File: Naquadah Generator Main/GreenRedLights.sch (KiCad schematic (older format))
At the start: 4 parts, among them J2 Conn_01x02, J5 Conn_01x02, Q1 BC337

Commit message: Before changing BOM
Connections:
- net labels added: +5V, GND
- net labels removed: 5V, VGND
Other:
- moved on the sheet: R33
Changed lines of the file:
@@
 $Descr A4 11693 8268
 encoding utf-8
-Sheet 11 14
+Sheet 9 10
 Title ""
 Date ""
@@
 $EndDescr
 Wire Wire Line
-	5450 4750 5400 4750
+	5450 4550 5450 4650
 Wire Wire Line
-	5450 4550 5450 4750
-Wire Wire Line
-	4650 4350 4850 4350
+	4650 4350 4750 4350
 Text HLabel 4650 4350 0    50   Input ~ 0
 SIGNAL
@@
 L Device:R R?
 U 1 1 5E9E70EB
-P 5000 4350
+P 4900 4350
 AR Path="/5E9E5DDE/5E9E70EB" Ref="R?"  Part="1"
 AR Path="/5E9E304D/5E9E70EB" Ref="R?"  Part="1"
@@
 AR Path="/5EA4676F/5E9E70EB" Ref="R33"  Part="1"
 AR Path="/5EA46A2B/5E9E70EB" Ref="R34"  Part="1"
-F 0 "R33" V 4793 4350 50  0000 C CNN
-F 1 "2.7k" V 4884 4350 50  0000 C CNN
-F 2 "Resistor_THT:R_Axial_DIN0207_L6.3mm_D2.5mm_P10.16mm_Horizontal" V 4930 4350 50  0001 C CNN
-F 3 "~" H 5000 4350 50  0001 C CNN
-	1    5000 4350
+F 0 "R33" V 4800 4350 50  0000 C CNN
+F 1 "2.7k" V 5000 4350 50  0000 C CNN
+F 2 "Resistor_THT:R_Axial_DIN0207_L6.3mm_D2.5mm_P10.16mm_Horizontal" V 4830 4350 50  0001 C CNN
+F 3 "~" H 4900 4350 50  0001 C CNN
+	1    4900 4350
 	0    1    1    0
 $EndComp
-Text GLabel 5400 4750 0    50   Input ~ 0
-VGND
 $Comp
 L Transistor_BJT:BC337 Q?
@@
 	1    0    0    -1
 $EndComp
-Text GLabel 5250 3650 0    50   Input ~ 0
-5V
 $Comp
 L Connector_Generic:Conn_01x02 J5
@@
 AR Path="/5EA4676F/5EAB251D" Ref="J6"  Part="1"
 AR Path="/5EA46A2B/5EAB251D" Ref="J?"  Part="1"
-F 0 "J6" H 6000 3700 50  0000 C CNN
-F 1 "Conn_01x02" H 6150 3800 50  0000 C CNN
+F 0 "J6" H 5900 3800 50  0000 L CNN
+F 1 "Conn_01x02" H 5900 3700 50  0000 L CNN
 F 2 "Connector_Wire:SolderWirePad_1x02_P3.81mm_Drill1.2mm" H 5800 3800 50  0001 C CNN
 F 3 "~" H 5800 3800 50  0001 C CNN
@@
 AR Path="/5EA4676F/5EA51394" Ref="J3"  Part="1"
 AR Path="/5EA46A2B/5EA51394" Ref="J4"  Part="1"
-F 0 "J3" H 5600 3800 50  0000 C CNN
-F 1 "Conn_01x02" H 5450 3900 50  0000 C CNN
+F 0 "J3" H 5650 3800 50  0000 R CNN
+F 1 "Conn_01x02" H 5650 3900 50  0000 R CNN
 F 2 "Connector_Wire:SolderWirePad_1x02_P3.81mm_Drill1.2mm" H 5100 3900 50  0001 C CNN
 F 3 "~" H 5100 3900 50  0001 C CNN
@@
 Wire Wire Line
 	5450 3900 5450 4150
-Text GLabel 5650 4050 2    50   Input ~ 0
-5V
 Wire Wire Line
-	5600 3900 5600 4050
+	5350 3750 5350 3800
 Wire Wire Line
-	5600 4050 5650 4050
+	5600 3900 5550 3900
 Wire Wire Line
-	5250 3650 5300 3650
+	5550 3900 5550 3750
+$Comp
+L power:+5V #PWR?
+U 1 1 5EC1DBF9
+P 5350 3750
+AR Path="/5EA45E37/5EC1DBF9" Ref="#PWR?"  Part="1"
+AR Path="/5EA4676F/5EC1DBF9" Ref="#PWR?"  Part="1"
+F 0 "#PWR?" H 5350 3600 50  0001 C CNN
+F 1 "+5V" H 5365 3923 50  0000 C CNN
+F 2 "" H 5350 3750 50  0001 C CNN
+F 3 "" H 5350 3750 50  0001 C CNN
+	1    5350 3750
+	1    0    0    -1
+$EndComp
+$Comp
+L power:+5V #PWR?
+U 1 1 5EC1E71E
+P 5550 3750
+AR Path="/5EA45E37/5EC1E71E" Ref="#PWR?"  Part="1"
+AR Path="/5EA4676F/5EC1E71E" Ref="#PWR?"  Part="1"
+F 0 "#PWR?" H 5550 3600 50  0001 C CNN
+F 1 "+5V" H 5565 3923 50  0000 C CNN
+F 2 "" H 5550 3750 50  0001 C CNN
+F 3 "" H 5550 3750 50  0001 C CNN
+	1    5550 3750
+	1    0    0    -1
+$EndComp
 Wire Wire Line
-	5300 3650 5300 3800
+	5350 3800 5300 3800
+$Comp
+L power:GND #PWR?
+U 1 1 5EC21498
+P 5450 4650
+AR Path="/5EA45E37/5EC21498" Ref="#PWR?"  Part="1"
+AR Path="/5EA4676F/5EC21498" Ref="#PWR?"  Part="1"
+F 0 "#PWR?" H 5450 4400 50  0001 C CNN
+F 1 "GND" H 5455 4477 50  0000 C CNN
+F 2 "" H 5450 4650 50  0001 C CNN
+F 3 "" H 5450 4650 50  0001 C CNN
+	1    5450 4650
+	1    0    0    -1
+$EndComp
+Wire Wire Line
+	5050 4350 5150 4350
 $EndSCHEMATC

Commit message: Changed name of libraries to remove underscore
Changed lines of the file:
@@
 $Descr A4 11693 8268
 encoding utf-8
-Sheet 9 10
+Sheet 9 11
 Title ""
 Date ""
@@
 AR Path="/5EA4676F/5E9E70EB" Ref="R33"  Part="1"
 AR Path="/5EA46A2B/5E9E70EB" Ref="R34"  Part="1"
-F 0 "R33" V 4800 4350 50  0000 C CNN
+AR Path="/5ED17BA0/5ED2A32F/5E9E70EB" Ref="R?"  Part="1"
+AR Path="/5ED17BA0/5ED2A36D/5E9E70EB" Ref="R?"  Part="1"
+F 0 "R?" V 4800 4350 50  0000 C CNN
 F 1 "2.7k" V 5000 4350 50  0000 C CNN
 F 2 "Resistor_THT:R_Axial_DIN0207_L6.3mm_D2.5mm_P10.16mm_Horizontal" V 4830 4350 50  0001 C CNN
@@
 AR Path="/5EA4676F/5EAB722E" Ref="Q2"  Part="1"
 AR Path="/5EA46A2B/5EAB722E" Ref="Q3"  Part="1"
-F 0 "Q2" H 5541 4396 50  0000 L CNN
+AR Path="/5ED17BA0/5ED2A32F/5EAB722E" Ref="Q?"  Part="1"
+AR Path="/5ED17BA0/5ED2A36D/5EAB722E" Ref="Q?"  Part="1"
+F 0 "Q?" H 5541 4396 50  0000 L CNN
 F 1 "BC337" H 5541 4305 50  0000 L CNN
 F 2 "Package_TO_SOT_THT:TO-92_Inline" H 5550 4275 50  0001 L CIN
@@
 AR Path="/5EA4676F/5EAB251D" Ref="J6"  Part="1"
 AR Path="/5EA46A2B/5EAB251D" Ref="J?"  Part="1"
-F 0 "J6" H 5900 3800 50  0000 L CNN
+AR Path="/5ED17BA0/5ED2A32F/5EAB251D" Ref="J?"  Part="1"
+AR Path="/5ED17BA0/5ED2A36D/5EAB251D" Ref="J?"  Part="1"
+F 0 "J?" H 5900 3800 50  0000 L CNN
 F 1 "Conn_01x02" H 5900 3700 50  0000 L CNN
 F 2 "Connector_Wire:SolderWirePad_1x02_P3.81mm_Drill1.2mm" H 5800 3800 50  0001 C CNN
@@
 AR Path="/5EA4676F/5EA51394" Ref="J3"  Part="1"
 AR Path="/5EA46A2B/5EA51394" Ref="J4"  Part="1"
-F 0 "J3" H 5650 3800 50  0000 R CNN
+AR Path="/5ED17BA0/5ED2A32F/5EA51394" Ref="J?"  Part="1"
+AR Path="/5ED17BA0/5ED2A36D/5EA51394" Ref="J?"  Part="1"
+F 0 "J?" H 5650 3800 50  0000 R CNN
 F 1 "Conn_01x02" H 5650 3900 50  0000 R CNN
 F 2 "Connector_Wire:SolderWirePad_1x02_P3.81mm_Drill1.2mm" H 5100 3900 50  0001 C CNN
@@
 AR Path="/5EA45E37/5EC1DBF9" Ref="#PWR?"  Part="1"
 AR Path="/5EA4676F/5EC1DBF9" Ref="#PWR?"  Part="1"
+AR Path="/5ED17BA0/5ED2A32F/5EC1DBF9" Ref="#PWR?"  Part="1"
+AR Path="/5ED17BA0/5ED2A36D/5EC1DBF9" Ref="#PWR?"  Part="1"
 F 0 "#PWR?" H 5350 3600 50  0001 C CNN
 F 1 "+5V" H 5365 3923 50  0000 C CNN
@@
 AR Path="/5EA45E37/5EC1E71E" Ref="#PWR?"  Part="1"
 AR Path="/5EA4676F/5EC1E71E" Ref="#PWR?"  Part="1"
+AR Path="/5ED17BA0/5ED2A32F/5EC1E71E" Ref="#PWR?"  Part="1"
+AR Path="/5ED17BA0/5ED2A36D/5EC1E71E" Ref="#PWR?"  Part="1"
 F 0 "#PWR?" H 5550 3600 50  0001 C CNN
 F 1 "+5V" H 5565 3923 50  0000 C CNN
@@
 AR Path="/5EA45E37/5EC21498" Ref="#PWR?"  Part="1"
 AR Path="/5EA4676F/5EC21498" Ref="#PWR?"  Part="1"
+AR Path="/5ED17BA0/5ED2A32F/5EC21498" Ref="#PWR?"  Part="1"
+AR Path="/5ED17BA0/5ED2A36D/5EC21498" Ref="#PWR?"  Part="1"
 F 0 "#PWR?" H 5450 4400 50  0001 C CNN
 F 1 "GND" H 5455 4477 50  0000 C CNN

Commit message: Partial Update
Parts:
- removed Q1: BC337, Package_TO_SOT_THT:TO-92_Inline, symbol Transistor_BJT:BC337
- added Q1: BCW65ALT1G, Package_TO_SOT_SMD:SOT-23, symbol Frequently_Used:BCW65ALT1G
- R30: renamed from R32; footprint Resistor_THT:R_Axial_DIN0207_L6.3mm_D2.5mm_P10.16mm_Horizontal -> Frequently_Used:0805_2012Metric_HandSolder
- renumbered J2 to J4
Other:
- moved on the sheet: J4, J5
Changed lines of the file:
@@
 $Descr A4 11693 8268
 encoding utf-8
-Sheet 9 11
+Sheet 10 11
 Title ""
 Date ""
@@
 AR Path="/5E9E5DE1/5E9E70EB" Ref="R?"  Part="1"
 AR Path="/5E9E4A6B/5E9E70EB" Ref="R?"  Part="1"
-AR Path="/5EA45E37/5E9E70EB" Ref="R32"  Part="1"
-AR Path="/5EA4676F/5E9E70EB" Ref="R33"  Part="1"
-AR Path="/5EA46A2B/5E9E70EB" Ref="R34"  Part="1"
-AR Path="/5ED17BA0/5ED2A32F/5E9E70EB" Ref="R?"  Part="1"
-AR Path="/5ED17BA0/5ED2A36D/5E9E70EB" Ref="R?"  Part="1"
-F 0 "R?" V 4800 4350 50  0000 C CNN
+AR Path="/5EA45E37/5E9E70EB" Ref="R?"  Part="1"
+AR Path="/5EA4676F/5E9E70EB" Ref="R?"  Part="1"
+AR Path="/5EA46A2B/5E9E70EB" Ref="R?"  Part="1"
+AR Path="/5ED17BA0/5ED2A32F/5E9E70EB" Ref="R30"  Part="1"
+AR Path="/5ED17BA0/5ED2A36D/5E9E70EB" Ref="R31"  Part="1"
+F 0 "R30" V 4800 4350 50  0000 C CNN
 F 1 "2.7k" V 5000 4350 50  0000 C CNN
-F 2 "Resistor_THT:R_Axial_DIN0207_L6.3mm_D2.5mm_P10.16mm_Horizontal" V 4830 4350 50  0001 C CNN
+F 2 "Frequently_Used:0805_2012Metric_HandSolder" V 4830 4350 50  0001 C CNN
 F 3 "~" H 4900 4350 50  0001 C CNN
 	1    4900 4350
@@
 $EndComp
 $Comp
-L Transistor_BJT:BC337 Q?
-U 1 1 5EAB722E
-P 5350 4350
-AR Path="/5E9E5DDE/5EAB722E" Ref="Q?"  Part="1"
-AR Path="/5E9E304D/5EAB722E" Ref="Q?"  Part="1"
-AR Path="/5E9D240B/5EAB722E" Ref="Q?"  Part="1"
-AR Path="/5E9E5DE1/5EAB722E" Ref="Q?"  Part="1"
-AR Path="/5E9E4A6B/5EAB722E" Ref="Q?"  Part="1"
-AR Path="/5EA45E37/5EAB722E" Ref="Q1"  Part="1"
-AR Path="/5EA4676F/5EAB722E" Ref="Q2"  Part="1"
-AR Path="/5EA46A2B/5EAB722E" Ref="Q3"  Part="1"
-AR Path="/5ED17BA0/5ED2A32F/5EAB722E" Ref="Q?"  Part="1"
-AR Path="/5ED17BA0/5ED2A36D/5EAB722E" Ref="Q?"  Part="1"
-F 0 "Q?" H 5541 4396 50  0000 L CNN
-F 1 "BC337" H 5541 4305 50  0000 L CNN
-F 2 "Package_TO_SOT_THT:TO-92_Inline" H 5550 4275 50  0001 L CIN
-F 3 "https://diotec.com/tl_files/diotec/files/pdf/datasheets/bc337.pdf" H 5350 4350 50  0001 L CNN
-	1    5350 4350
+L Connector_Generic:Conn_01x02 J?
+U 1 1 5EAB251D
+P 5800 3750
+AR Path="/5EA45E37/5EAB251D" Ref="J?"  Part="1"
+AR Path="/5EA4676F/5EAB251D" Ref="J?"  Part="1"
+AR Path="/5EA46A2B/5EAB251D" Ref="J?"  Part="1"
+AR Path="/5ED17BA0/5ED2A32F/5EAB251D" Ref="J5"  Part="1"
+AR Path="/5ED17BA0/5ED2A36D/5EAB251D" Ref="J7"  Part="1"
+F 0 "J5" H 5900 3750 50  0000 L CNN
+F 1 "Conn_01x02" H 5900 3650 50  0000 L CNN
+F 2 "Connector_Wire:SolderWirePad_1x02_P3.81mm_Drill1.2mm" H 5800 3750 50  0001 C CNN
+F 3 "~" H 5800 3750 50  0001 C CNN
+	1    5800 3750
 	1    0    0    -1
 $EndComp
 $Comp
-L Connector_Generic:Conn_01x02 J5
-U 1 1 5EAB251D
-P 5800 3800
-AR Path="/5EA45E37/5EAB251D" Ref="J5"  Part="1"
-AR Path="/5EA4676F/5EAB251D" Ref="J6"  Part="1"
-AR Path="/5EA46A2B/5EAB251D" Ref="J?"  Part="1"
-AR Path="/5ED17BA0/5ED2A32F/5EAB251D" Ref="J?"  Part="1"
-AR Path="/5ED17BA0/5ED2A36D/5EAB251D" Ref="J?"  Part="1"
-F 0 "J?" H 5900 3800 50  0000 L CNN
-F 1 "Conn_01x02" H 5900 3700 50  0000 L CNN
-F 2 "Connector_Wire:SolderWirePad_1x02_P3.81mm_Drill1.2mm" H 5800 3800 50  0001 C CNN
-F 3 "~" H 5800 3800 50  0001 C CNN
-	1    5800 3800
-	1    0    0    -1
-$EndComp
-$Comp
-L Connector_Generic:Conn_01x02 J2
+L Connector_Generic:Conn_01x02 J?
 U 1 1 5EA51394
-P 5100 3900
-AR Path="/5EA45E37/5EA51394" Ref="J2"  Part="1"
-AR Path="/5EA4676F/5EA51394" Ref="J3"  Part="1"
-AR Path="/5EA46A2B/5EA51394" Ref="J4"  Part="1"
-AR Path="/5ED17BA0/5ED2A32F/5EA51394" Ref="J?"  Part="1"
-AR Path="/5ED17BA0/5ED2A36D/5EA51394" Ref="J?"  Part="1"
-F 0 "J?" H 5650 3800 50  0000 R CNN
-F 1 "Conn_01x02" H 5650 3900 50  0000 R CNN
-F 2 "Connector_Wire:SolderWirePad_1x02_P3.81mm_Drill1.2mm" H 5100 3900 50  0001 C CNN
-F 3 "~" H 5100 3900 50  0001 C CNN
-	1    5100 3900
+P 5100 3850
+AR Path="/5EA45E37/5EA51394" Ref="J?"  Part="1"
+AR Path="/5EA4676F/5EA51394" Ref="J?"  Part="1"
+AR Path="/5EA46A2B/5EA51394" Ref="J?"  Part="1"
+AR Path="/5ED17BA0/5ED2A32F/5EA51394" Ref="J4"  Part="1"
+AR Path="/5ED17BA0/5ED2A36D/5EA51394" Ref="J6"  Part="1"
+F 0 "J4" H 5650 3750 50  0000 R CNN
+F 1 "Conn_01x02" H 5650 3850 50  0000 R CNN
+F 2 "Connector_Wire:SolderWirePad_1x02_P3.81mm_Drill1.2mm" H 5100 3850 50  0001 C CNN
+F 3 "~" H 5100 3850 50  0001 C CNN
+	1    5100 3850
 	-1   0    0    1
 $EndComp
 Wire Wire Line
-	5600 3800 5450 3800
+	5600 3750 5450 3750
 Wire Wire Line
-	5450 3800 5450 3900
+	5450 3750 5450 3850
 Wire Wire Line
-	5300 3900 5450 3900
-Connection ~ 5450 3900
+	5300 3850 5450 3850
+Connection ~ 5450 3850
 Wire Wire Line
-	5450 3900 5450 4150
+	5450 3850 5450 4150
 Wire Wire Line
-	5350 3750 5350 3800
+	5350 3700 5350 3750
 Wire Wire Line
-	5600 3900 5550 3900
+	5600 3850 5550 3850
 Wire Wire Line
-	5550 3900 5550 3750
+	5550 3850 5550 3700
 $Comp
 L power:+5V #PWR?
 U 1 1 5EC1DBF9
-P 5350 3750
+P 5350 3700
 AR Path="/5EA45E37/5EC1DBF9" Ref="#PWR?"  Part="1"
 AR Path="/5EA4676F/5EC1DBF9" Ref="#PWR?"  Part="1"
-AR Path="/5ED17BA0/5ED2A32F/5EC1DBF9" Ref="#PWR?"  Part="1"
-AR Path="/5ED17BA0/5ED2A36D/5EC1DBF9" Ref="#PWR?"  Part="1"
-F 0 "#PWR?" H 5350 3600 50  0001 C CNN
-F 1 "+5V" H 5365 3923 50  0000 C CNN
-F 2 "" H 5350 3750 50  0001 C CNN
-F 3 "" H 5350 3750 50  0001 C CNN
-	1    5350 3750
+AR Path="/5ED17BA0/5ED2A32F/5EC1DBF9" Ref="#PWR046"  Part="1"
+AR Path="/5ED17BA0/5ED2A36D/5EC1DBF9" Ref="#PWR049"  Part="1"
+F 0 "#PWR046" H 5350 3550 50  0001 C CNN
+F 1 "+5V" H 5365 3873 50  0000 C CNN
+F 2 "" H 5350 3700 50  0001 C CNN
+F 3 "" H 5350 3700 50  0001 C CNN
+	1    5350 3700
 	1    0    0    -1
 $EndComp
@@
 L power:+5V #PWR?
 U 1 1 5EC1E71E
-P 5550 3750
+P 5550 3700
 AR Path="/5EA45E37/5EC1E71E" Ref="#PWR?"  Part="1"
 AR Path="/5EA4676F/5EC1E71E" Ref="#PWR?"  Part="1"
-AR Path="/5ED17BA0/5ED2A32F/5EC1E71E" Ref="#PWR?"  Part="1"
-AR Path="/5ED17BA0/5ED2A36D/5EC1E71E" Ref="#PWR?"  Part="1"
-F 0 "#PWR?" H 5550 3600 50  0001 C CNN
-F 1 "+5V" H 5565 3923 50  0000 C CNN
-F 2 "" H 5550 3750 50  0001 C CNN
-F 3 "" H 5550 3750 50  0001 C CNN
-	1    5550 3750
+AR Path="/5ED17BA0/5ED2A32F/5EC1E71E" Ref="#PWR048"  Part="1"
+AR Path="/5ED17BA0/5ED2A36D/5EC1E71E" Ref="#PWR051"  Part="1"
+F 0 "#PWR048" H 5550 3550 50  0001 C CNN
+F 1 "+5V" H 5565 3873 50  0000 C CNN
+F 2 "" H 5550 3700 50  0001 C CNN
+F 3 "" H 5550 3700 50  0001 C CNN
+	1    5550 3700
 	1    0    0    -1
 $EndComp
 Wire Wire Line
-	5350 3800 5300 3800
+	5350 3750 5300 3750
 $Comp
 L power:GND #PWR?
@@
 AR Path="/5EA45E37/5EC21498" Ref="#PWR?"  Part="1"
 AR Path="/5EA4676F/5EC21498" Ref="#PWR?"  Part="1"
-AR Path="/5ED17BA0/5ED2A32F/5EC21498" Ref="#PWR?"  Part="1"
-AR Path="/5ED17BA0/5ED2A36D/5EC21498" Ref="#PWR?"  Part="1"
-F 0 "#PWR?" H 5450 4400 50  0001 C CNN
+AR Path="/5ED17BA0/5ED2A32F/5EC21498" Ref="#PWR047"  Part="1"
+AR Path="/5ED17BA0/5ED2A36D/5EC21498" Ref="#PWR050"  Part="1"
+F 0 "#PWR047" H 5450 4400 50  0001 C CNN
 F 1 "GND" H 5455 4477 50  0000 C CNN
 F 2 "" H 5450 4650 50  0001 C CNN
@@
 Wire Wire Line
 	5050 4350 5150 4350
+$Comp
+L Frequently_Used:BCW65ALT1G Q1
+U 1 1 5EE732B9
+P 5350 4350
+AR Path="/5ED17BA0/5ED2A36D/5EE732B9" Ref="Q1"  Part="1"
+AR Path="/5ED17BA0/5ED2A32F/5EE732B9" Ref="Q2"  Part="1"
+F 0 "Q2" H 5541 4396 50  0000 L CNN
+F 1 "BCW65ALT1G" H 5541 4305 50  0000 L CNN
+F 2 "Package_TO_SOT_SMD:SOT-23" H 5400 3700 50  0001 C CIN
+F 3 "https://www.onsemi.com/pub/Collateral/BCW65ALT1-D.PDF" H 5350 4350 50  0001 L CNN
+F 4 "ON Semiconductor" H 5400 3600 50  0001 C CNN "Manufacturer Name"
+F 5 "BCW65ALT1G" H 5400 3900 50  0001 C CNN "Manufacturer Part No."
+F 6 "488-BCW65ALT1GCT-ND" H 5400 3800 50  0001 C CNN "Digikey Part No."
+	1    5350 4350
+	1    0    0    -1
+$EndComp
 $EndSCHEMATC

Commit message: Resize to correct for scale
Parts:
- removed Q1: BCW65ALT1G, Package_TO_SOT_SMD:SOT-23, symbol Frequently_Used:BCW65ALT1G
- removed R30: 2.7k, Frequently_Used:0805_2012Metric_HandSolder, symbol Device:R
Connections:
- net labels added: COLLECTOR
- net labels removed: GND, SIGNAL
- wire segments 11 -> 9
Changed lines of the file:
@@
 $Descr A4 11693 8268
 encoding utf-8
-Sheet 10 11
+Sheet 9 10
 Title ""
 Date ""
@@
 $EndDescr
 Wire Wire Line
-	5450 4550 5450 4650
-Wire Wire Line
-	4650 4350 4750 4350
-Text HLabel 4650 4350 0    50   Input ~ 0
-SIGNAL
-$Comp
-L Device:R R?
-U 1 1 5E9E70EB
-P 4900 4350
-AR Path="/5E9E5DDE/5E9E70EB" Ref="R?"  Part="1"
-AR Path="/5E9E304D/5E9E70EB" Ref="R?"  Part="1"
-AR Path="/5E9D240B/5E9E70EB" Ref="R?"  Part="1"
-AR Path="/5E9E5DE1/5E9E70EB" Ref="R?"  Part="1"
-AR Path="/5E9E4A6B/5E9E70EB" Ref="R?"  Part="1"
-AR Path="/5EA45E37/5E9E70EB" Ref="R?"  Part="1"
-AR Path="/5EA4676F/5E9E70EB" Ref="R?"  Part="1"
-AR Path="/5EA46A2B/5E9E70EB" Ref="R?"  Part="1"
-AR Path="/5ED17BA0/5ED2A32F/5E9E70EB" Ref="R30"  Part="1"
-AR Path="/5ED17BA0/5ED2A36D/5E9E70EB" Ref="R31"  Part="1"
-F 0 "R30" V 4800 4350 50  0000 C CNN
-F 1 "2.7k" V 5000 4350 50  0000 C CNN
-F 2 "Frequently_Used:0805_2012Metric_HandSolder" V 4830 4350 50  0001 C CNN
-F 3 "~" H 4900 4350 50  0001 C CNN
-	1    4900 4350
-	0    1    1    0
-$EndComp
+	5350 4150 5450 4150
+Text HLabel 5350 4150 0    50   Input ~ 0
+COLLECTOR
 $Comp
 L Connector_Generic:Conn_01x02 J?
@@
 Wire Wire Line
 	5350 3750 5300 3750
-$Comp
-L power:GND #PWR?
-U 1 1 5EC21498
-P 5450 4650
-AR Path="/5EA45E37/5EC21498" Ref="#PWR?"  Part="1"
-AR Path="/5EA4676F/5EC21498" Ref="#PWR?"  Part="1"
-AR Path="/5ED17BA0/5ED2A32F/5EC21498" Ref="#PWR047"  Part="1"
-AR Path="/5ED17BA0/5ED2A36D/5EC21498" Ref="#PWR050"  Part="1"
-F 0 "#PWR047" H 5450 4400 50  0001 C CNN
-F 1 "GND" H 5455 4477 50  0000 C CNN
-F 2 "" H 5450 4650 50  0001 C CNN
-F 3 "" H 5450 4650 50  0001 C CNN
-	1    5450 4650
-	1    0    0    -1
-$EndComp
-Wire Wire Line
-	5050 4350 5150 4350
-$Comp
-L Frequently_Used:BCW65ALT1G Q1
-U 1 1 5EE732B9
-P 5350 4350
-AR Path="/5ED17BA0/5ED2A36D/5EE732B9" Ref="Q1"  Part="1"
-AR Path="/5ED17BA0/5ED2A32F/5EE732B9" Ref="Q2"  Part="1"
-F 0 "Q2" H 5541 4396 50  0000 L CNN
-F 1 "BCW65ALT1G" H 5541 4305 50  0000 L CNN
-F 2 "Package_TO_SOT_SMD:SOT-23" H 5400 3700 50  0001 C CIN
-F 3 "https://www.onsemi.com/pub/Collateral/BCW65ALT1-D.PDF" H 5350 4350 50  0001 L CNN
-F 4 "ON Semiconductor" H 5400 3600 50  0001 C CNN "Manufacturer Name"
-F 5 "BCW65ALT1G" H 5400 3900 50  0001 C CNN "Manufacturer Part No."
-F 6 "488-BCW65ALT1GCT-ND" H 5400 3800 50  0001 C CNN "Digikey Part No."
-	1    5350 4350
-	1    0    0    -1
-$EndComp
 $EndSCHEMATC

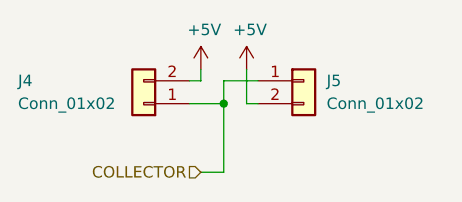
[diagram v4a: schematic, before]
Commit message: Updates to PCB Mount
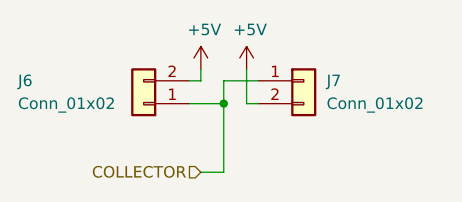
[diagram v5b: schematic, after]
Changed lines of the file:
@@
 AR Path="/5ED17BA0/5ED2A32F/5EAB251D" Ref="J5"  Part="1"
 AR Path="/5ED17BA0/5ED2A36D/5EAB251D" Ref="J7"  Part="1"
-F 0 "J5" H 5900 3750 50  0000 L CNN
+F 0 "J7" H 5900 3750 50  0000 L CNN
 F 1 "Conn_01x02" H 5900 3650 50  0000 L CNN
 F 2 "Connector_Wire:SolderWirePad_1x02_P3.81mm_Drill1.2mm" H 5800 3750 50  0001 C CNN
@@
 AR Path="/5ED17BA0/5ED2A32F/5EA51394" Ref="J4"  Part="1"
 AR Path="/5ED17BA0/5ED2A36D/5EA51394" Ref="J6"  Part="1"
-F 0 "J4" H 5650 3750 50  0000 R CNN
+F 0 "J6" H 5650 3750 50  0000 R CNN
 F 1 "Conn_01x02" H 5650 3850 50  0000 R CNN
 F 2 "Connector_Wire:SolderWirePad_1x02_P3.81mm_Drill1.2mm" H 5100 3850 50  0001 C CNN
@@
 AR Path="/5ED17BA0/5ED2A32F/5EC1DBF9" Ref="#PWR046"  Part="1"
 AR Path="/5ED17BA0/5ED2A36D/5EC1DBF9" Ref="#PWR049"  Part="1"
-F 0 "#PWR046" H 5350 3550 50  0001 C CNN
+F 0 "#PWR049" H 5350 3550 50  0001 C CNN
 F 1 "+5V" H 5365 3873 50  0000 C CNN
 F 2 "" H 5350 3700 50  0001 C CNN
@@
 AR Path="/5ED17BA0/5ED2A32F/5EC1E71E" Ref="#PWR048"  Part="1"
 AR Path="/5ED17BA0/5ED2A36D/5EC1E71E" Ref="#PWR051"  Part="1"
-F 0 "#PWR048" H 5550 3550 50  0001 C CNN
+F 0 "#PWR051" H 5550 3550 50  0001 C CNN
 F 1 "+5V" H 5565 3873 50  0000 C CNN
 F 2 "" H 5550 3700 50  0001 C CNN
